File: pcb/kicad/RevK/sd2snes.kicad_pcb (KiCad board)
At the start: 2 copper layers, 101.5 x 83 mm, 148 parts, among them J101 SNESCART_EXT, J411 Hirose DM1AA, J421 USB Mini-B SMT, P113 CONN_1, P401 CONN_7X2, P402 CONN_2, P403 CONN_2, P404 CONN_3X2, Q101 2N2222A, Q301 IRLML6402PbF, Q511 2N2222A, U101 74ALVC164245DGG, U102 74ALVC164245DGG, U103 74ALVC164245DGG, U201 XC3S400-PQ208, U230 TS9222, U301 MIC23250-S4YMT, U311 MCP1824-1802E/OT, U321 MCP1824-2502E/OT, U331 PIC12F629-I/P, U341 CS4344, U401 LPC1754, U501 MT45W8MW16, U511 CY62148EV30-ZSXI, X401 12MHz, X402 32.768kHz

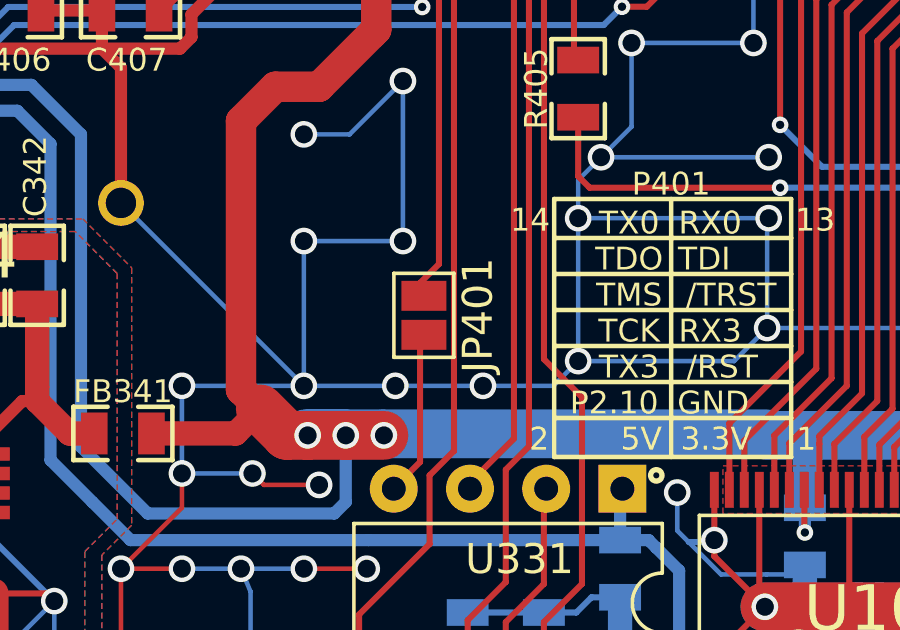
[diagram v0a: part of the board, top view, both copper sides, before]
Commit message: Fix tracing again, fixing other stuff in Schema
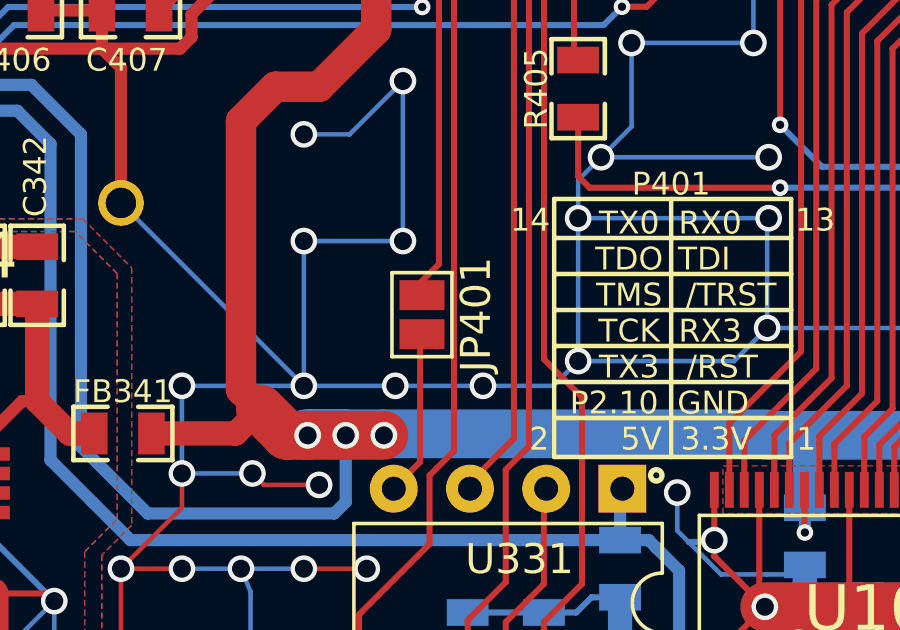
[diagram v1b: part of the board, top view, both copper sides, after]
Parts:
- moved JP401 0.07 mm to (121.8, 107.4)
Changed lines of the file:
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@@
   )
   (layers
-    (0 Component signal hide)
-    (31 Copper signal)
+    (0 Component signal)
+    (31 Copper signal hide)
     (32 B.Adhes user hide)
     (33 F.Adhes user hide)
@@
   )
   (module Jumper:SolderJumper-2_P1.3mm_Open_Pad1.0x1.5mm (layer Component)
-    (at 121.8565 107.3785 270)
+    (at 121.793 107.3554 270)
     (descr "SMD Solder Jumper, 1x1.5mm Pads, 0.3mm gap, open")
     (tags "solder jumper open")
